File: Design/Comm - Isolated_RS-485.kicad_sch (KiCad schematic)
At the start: 50 parts, among them J12 RS-485, J13 RS-485, U7 ISO3082DWR, U8 ISO3082DWR

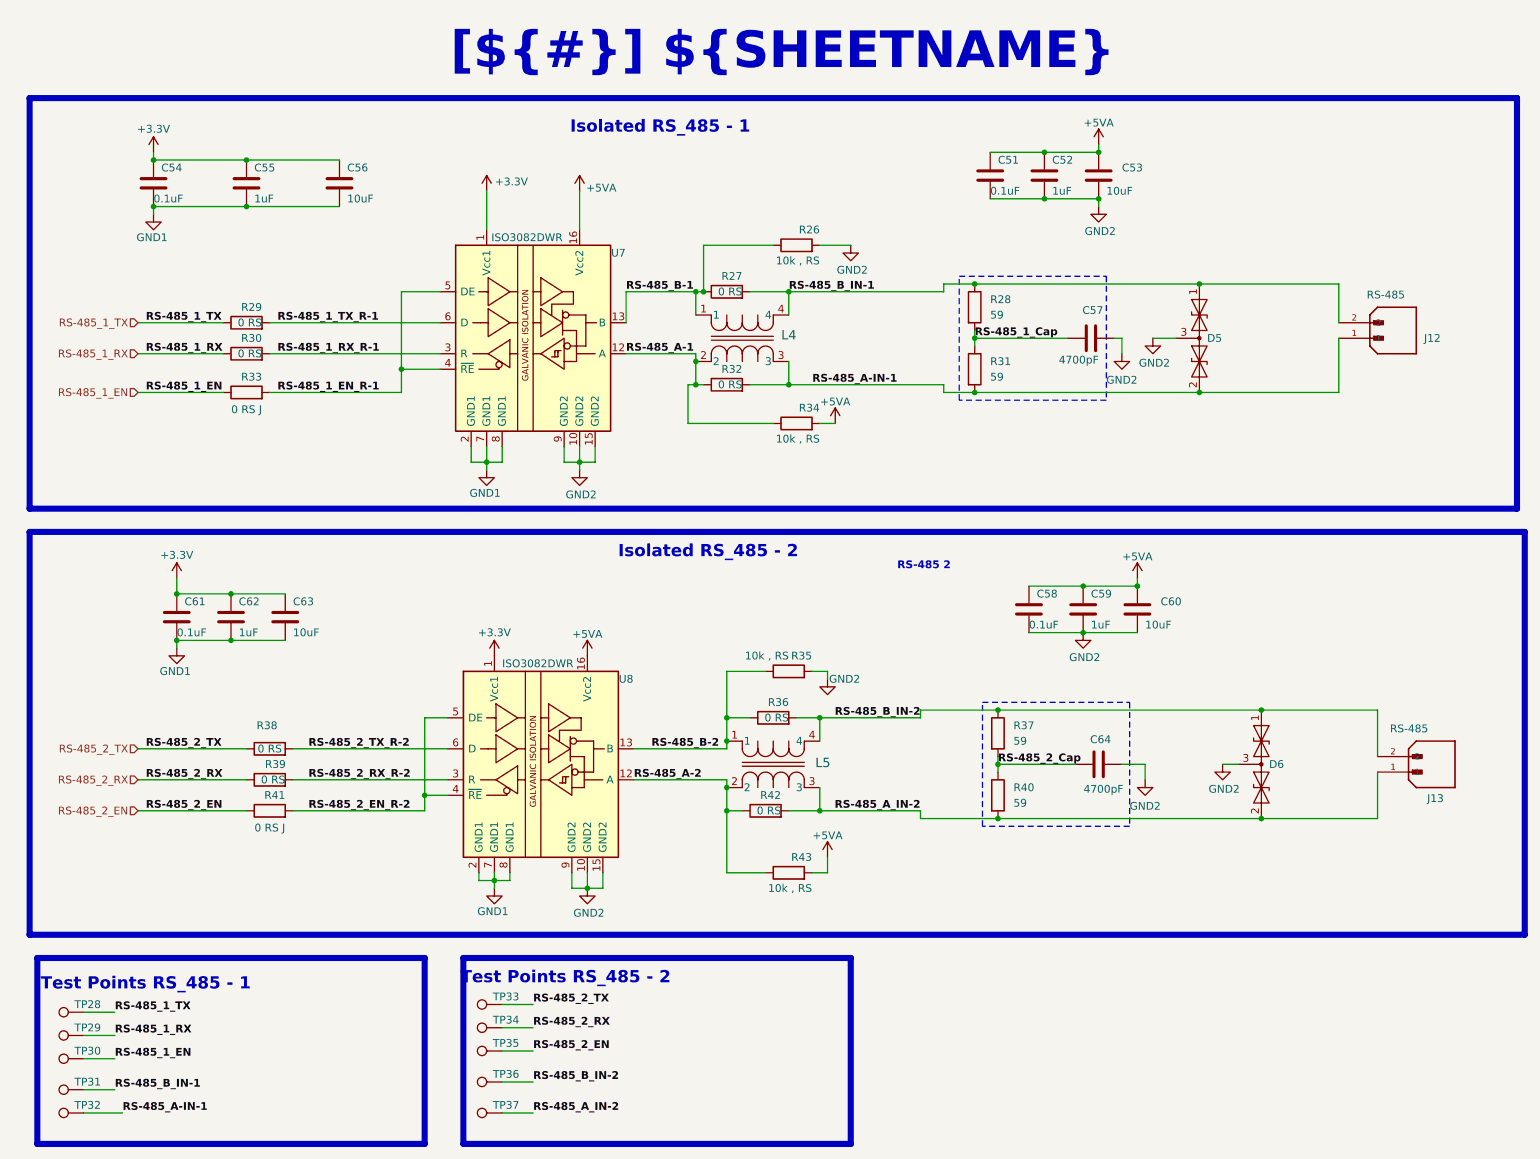
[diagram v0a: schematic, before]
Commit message: new Design for Prototyping
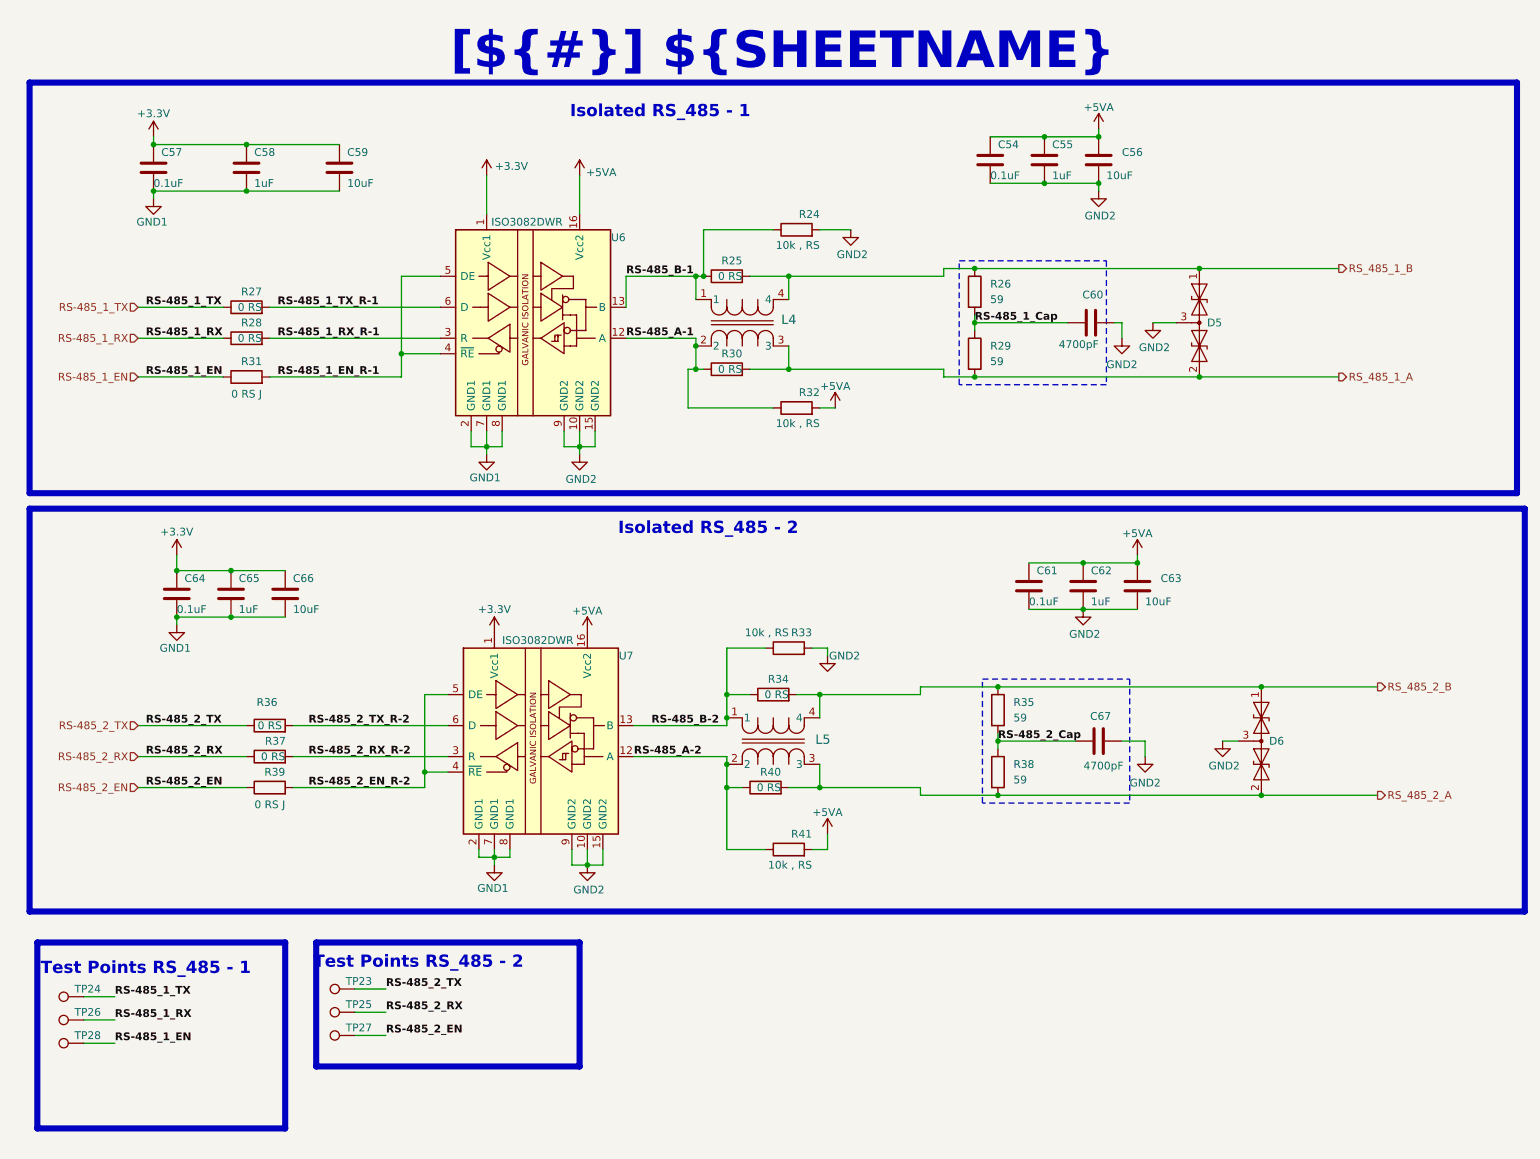
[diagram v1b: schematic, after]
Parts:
- removed J12, J13: RS-485, 0530480210_2pin_P1.25_PicoBlade:MOLEX_530480210, symbol 0530480210_2pin_P1.25_PicoBlade:530480210
- removed TP31, TP32, TP36, TP37: Test_point, Test_point:Test_point, symbol Test_point:Test_point
- renumbered C51 to C54, C52 to C55, C53 to C56, C54 to C57, C55 to C58, C56 to C59, C57 to C60, C58 to C61, C59 to C62, C60 to C63, C61 to C64, C62 to C65, C63 to C66, C64 to C67, R26 to R24, R27 to R25, R28 to R26, R29 to R27, R30 to R28, R31 to R29, R32 to R30, R33 to R31, R34 to R32, R35 to R33, R36 to R34, R37 to R35, R38 to R36, R39 to R37, R40 to R38, R41 to R39, R42 to R40, R43 to R41, TP33 to TP23, TP28 to TP24, TP34 to TP25, TP29 to TP26, TP35 to TP27, TP30 to TP28, U7 to U6, U8 to U7
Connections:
- net RS-485_A-IN-1 renamed RS_485_1_A
- net RS-485_A_IN-2 renamed RS_485_2_A
- net RS-485_B_IN-1 renamed RS_485_1_B
- net RS-485_B_IN-2 renamed RS_485_2_B
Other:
- note removed: "RS-485 2"
- title: Rapid-Core -> (none)
- moved on the sheet: C54, C55, C56, C57, C58, C59, C60, C61, C62, C63, C64, C65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
